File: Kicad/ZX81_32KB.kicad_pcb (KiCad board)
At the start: 2 copper layers, 25 x 44 mm, 4 parts, among them IC1 CY62256NLL-55SNXI, J1 Conn_01x14_Pin, J2 Conn_01x14_Pin, J3 Conn_01x04_Pin

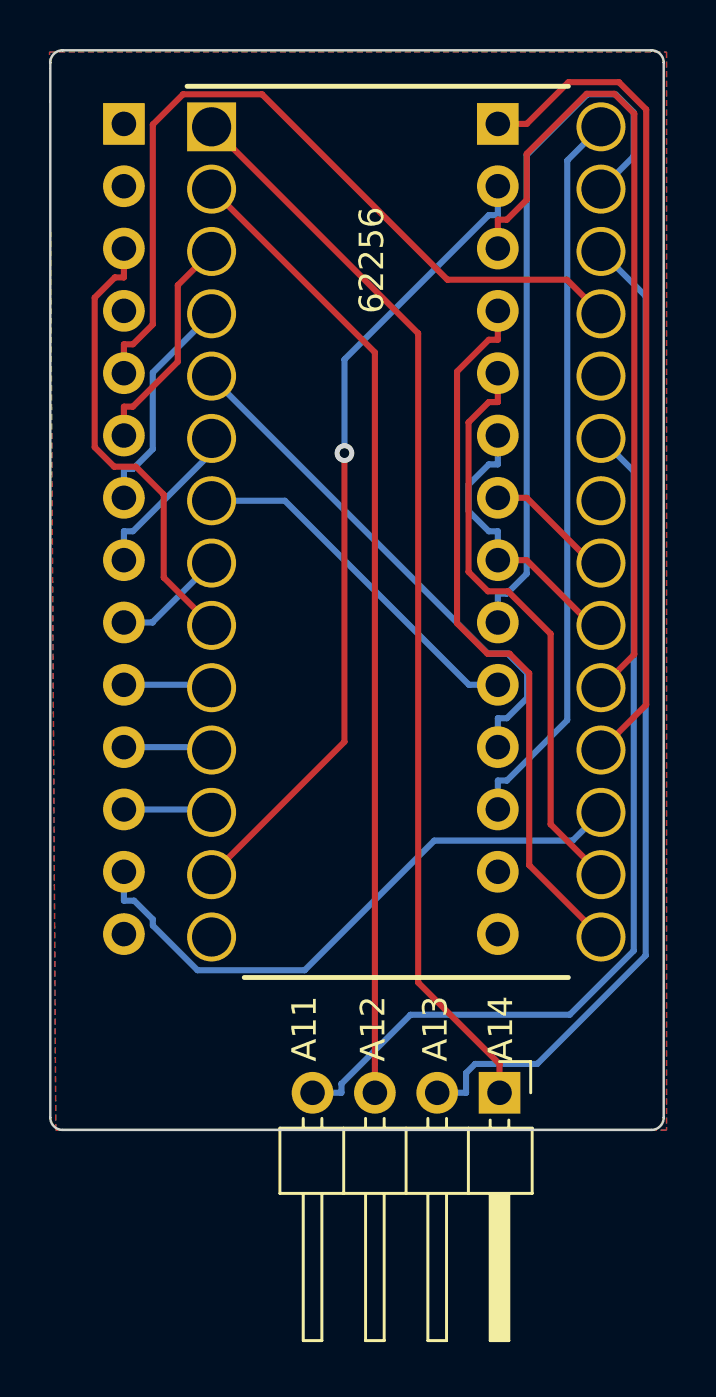
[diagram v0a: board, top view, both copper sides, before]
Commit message: Refinements
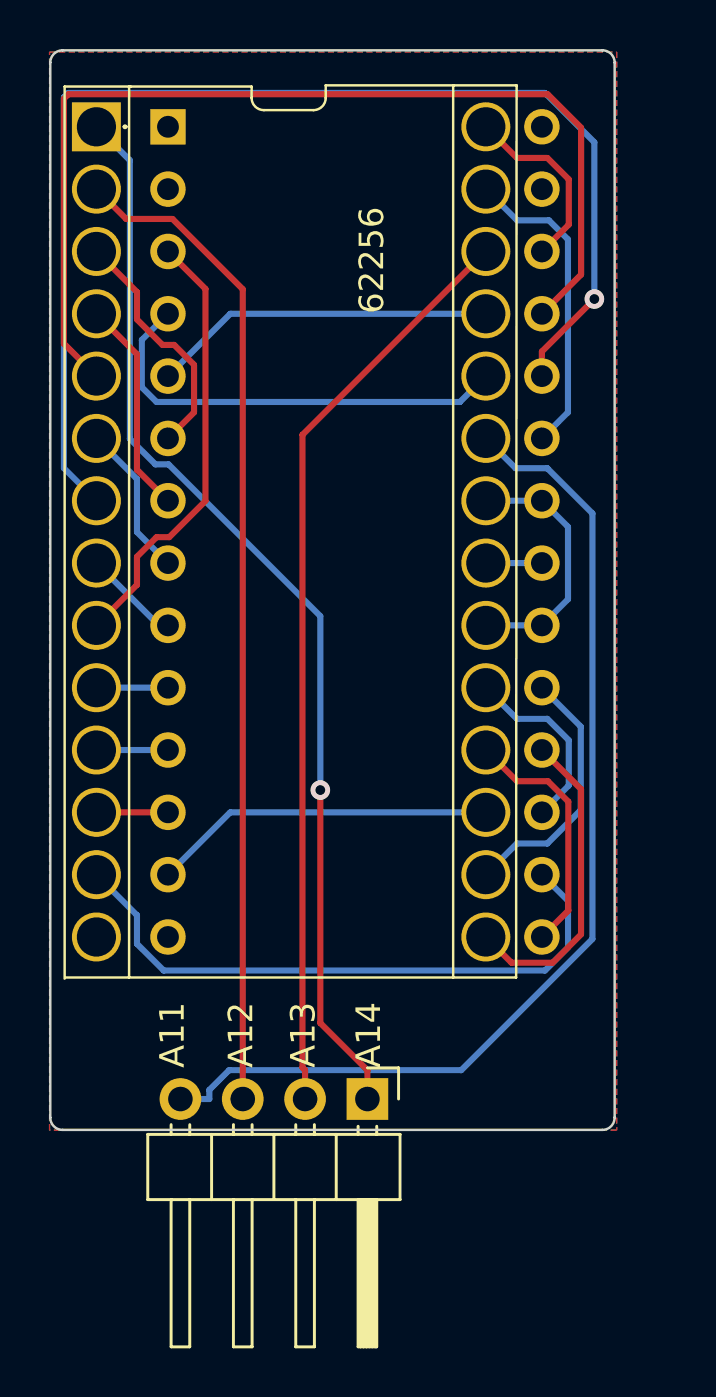
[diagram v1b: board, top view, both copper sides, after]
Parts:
- removed J1, J2: Conn_01x14_Pin, Connector_PinHeader_2.54mm:PinHeader_1x14_P2.54mm_Vertical
- added J4: 828-AG11D-LF, CluelessEngineer:828AG11DLF, F.Cu at (145.8, 55.1)
- moved J3 5.39 mm to (153.9, 94.7)
- moved IC1 4.69 mm to (150.8, 71.6)
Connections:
- IC1 pad 22: /GND -> /~{RAMCS}
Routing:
- net /A03: track 14.8 -> 49.9 mm, vias 0 -> 1
- net /D7: track 34.3 -> 7.66 mm
- net /D6: track 34.1 -> 10.2 mm
- net /+5V: track 29.8 -> 7.66 mm
- net /A05: track 21.6 -> 41.8 mm
- net /A08: track 33.3 -> 14.0 mm
- net /A09: track 0.00 -> 18.1 mm
- net /D3: track 29.4 -> 13.0 mm
- net /~{WR}: track 29.1 -> 12.7 mm
- net /D4: track 23.9 -> 10.6 mm
- net /D5: track 24.6 -> 14.0 mm
- net /D2: track 33.1 -> 25.3 mm, vias 1 -> 0
- net /A11: track 37.1 -> 42.7 mm
- net /A13: track 40.7 -> 37.7 mm
- net /A10: track 5.30 -> 2.29 mm
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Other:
- board size 25 x 44 mm -> 23 x 44 mm
- board text added: "ZX81/TS1000 32KB RAM Board for vLA81 Designed in Port Macquarie, Australia Brett Hallen, Sept 2023 youtube.com/@brfff"
- board text removed: "ZX81/TS1000 32KB RAM Board Designed in Port Macquarie, Australia Brett Hallen, Sept 2023 youtube.com/@brfff"
